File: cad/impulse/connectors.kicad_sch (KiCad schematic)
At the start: 29 parts, among them J1 Screw_Terminal_01x02, J10 Screw_Terminal_01x02, J2 Screw_Terminal_01x02, J3 Conn_01x08, J4 Conn_01x08, J5 Conn_01x08, J6 Screw_Terminal_01x02, J7 GT-USB-7010ASV, J8 Screw_Terminal_01x02, J9 Screw_Terminal_01x02, Q2 Q_NMOS_DGS, Q3 Q_NMOS_DGS, Q4 Q_NMOS_DGS, Q5 Q_NMOS_DGS, U3 USBLC6-2SC6

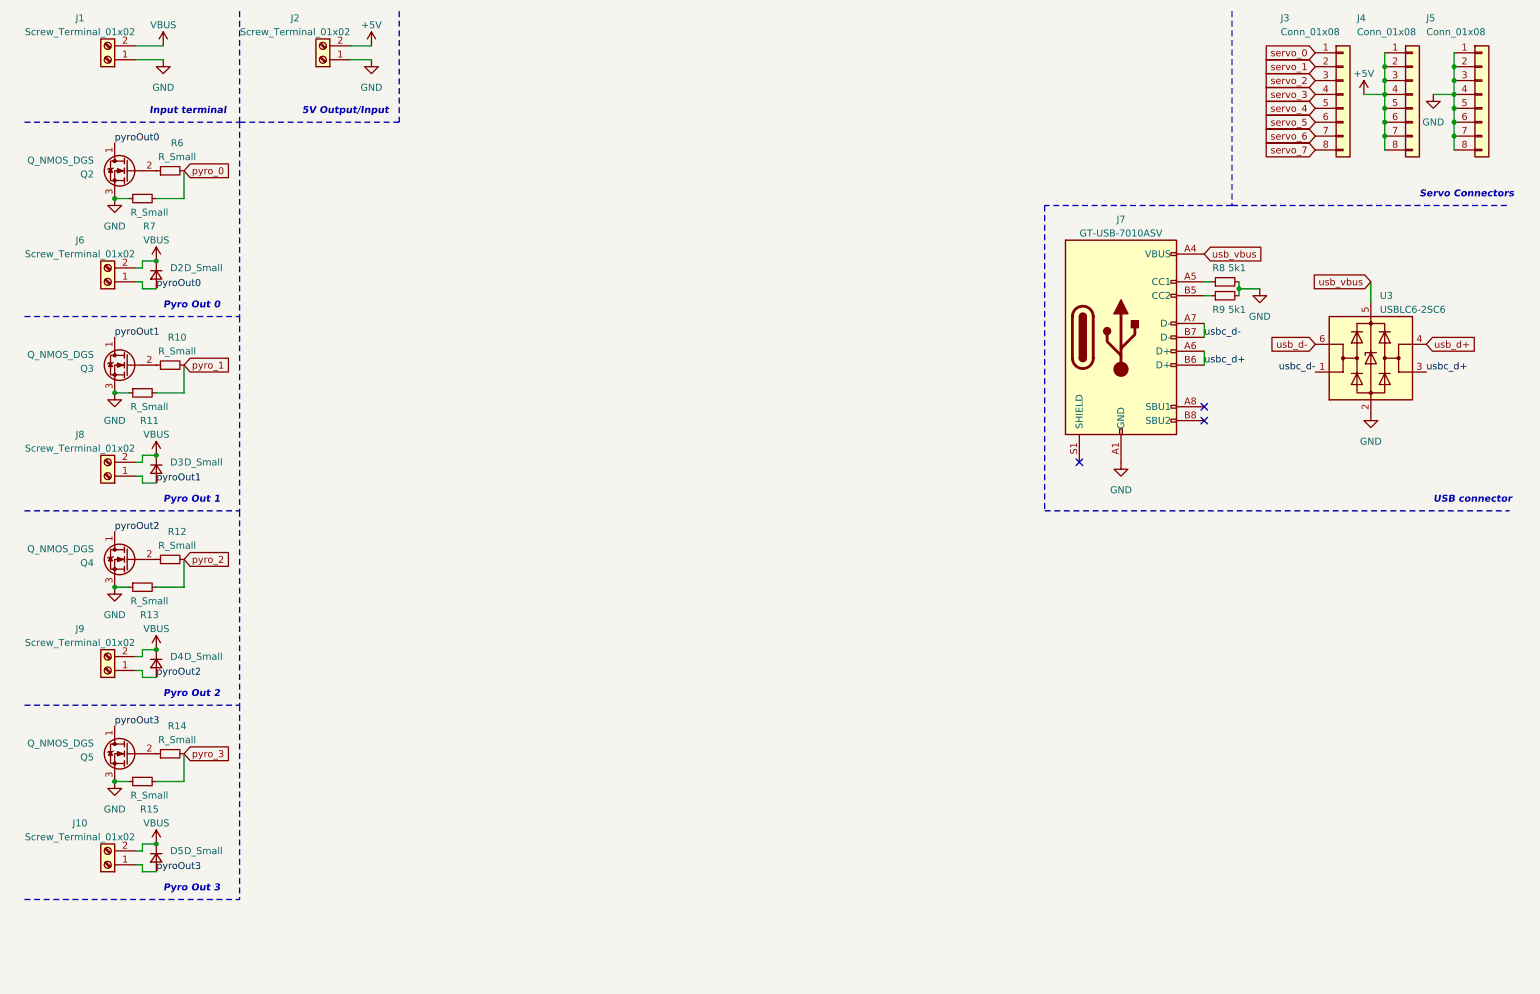
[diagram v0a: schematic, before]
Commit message: Finnished the design.
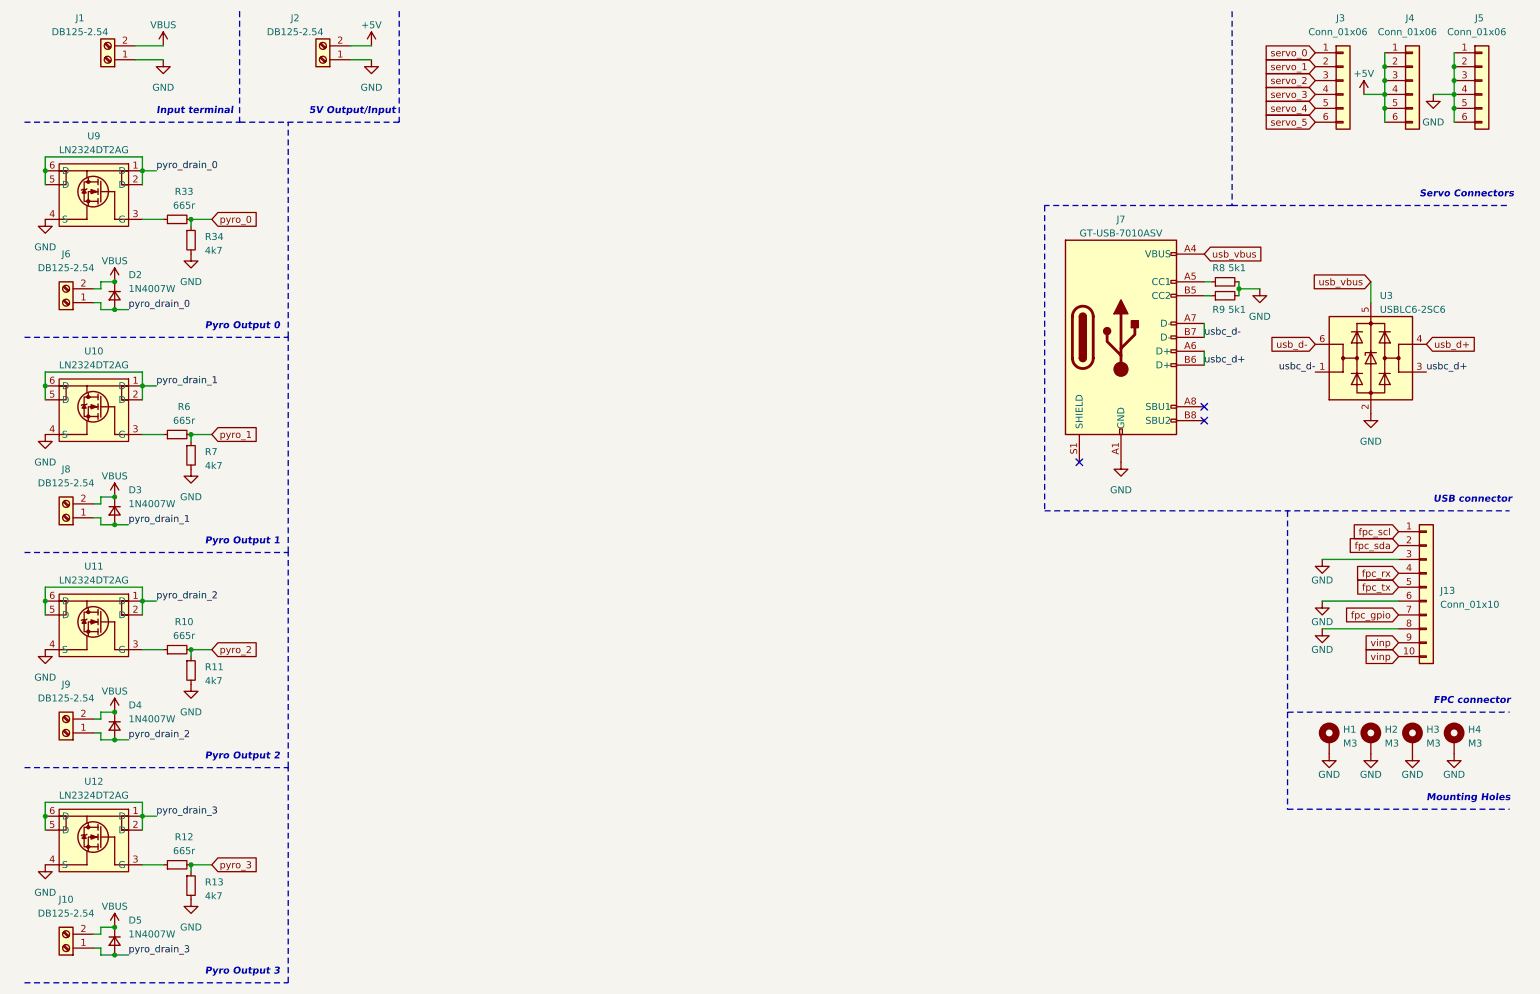
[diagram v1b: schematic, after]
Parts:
- removed J3, J4, J5: Conn_01x08, Connector_RJ:RJ45_Amphenol_54602-x08_Horizontal, symbol Connector_Generic:Conn_01x08
- removed Q2, Q3, Q4, Q5: Q_NMOS_DGS, symbol Device:Q_NMOS_DGS
- removed R14, R15: R_Small, symbol Device:R_Small
- added H1, H2, H3, H4: M3, symbol Mechanical:MountingHole_Pad
- added J13: Conn_01x10, symbol Connector_Generic:Conn_01x10
- added J3, J4, J5: Conn_01x06, symbol Connector_Generic:Conn_01x06
- added R33: 665r, symbol Device:R_Small
- added R34: 4k7, symbol Device:R_Small
- added U10, U11, U12, U9: LN2324DT2AG, symbol impulse:LN2324DT2AG
- D2, D3, D4, D5: value D_Small -> 1N4007W
- J1, J10, J2, J6, J8, J9: value Screw_Terminal_01x02 -> DB125-2.54
- R10, R12, R6: value R_Small -> 665r
- R11, R13, R7: value R_Small -> 4k7
- U3: footprint Package_TO_SOT_SMD:SOT-23-6 -> (none)
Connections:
- net +5V: now also J4.1 (Pin_1), J4.2 (Pin_2), J4.3 (Pin_3), J4.4 (Pin_4), J4.5 (Pin_5), J4.6 (Pin_6)
- net GND: now also R11.2, R13.2, R7.2, H1.1, H2.1, H3.1, H4.1, J13.3 (Pin_3), J13.6 (Pin_6), J13.8 (Pin_8), J5.1 (Pin_1), J5.2 (Pin_2), J5.3 (Pin_3), J5.4 (Pin_4), J5.5 (Pin_5), J5.6 (Pin_6), R34.2, U10.4 (S), U11.4 (S), U12.4 (S), U9.4 (S); no longer R11.1, R13.1, R7.1
- net pyro_0: now also R33.2, R34.1; no longer R6.2, R7.2
- net pyro_1: now also R6.2, R7.1; no longer R10.2, R11.2
- net pyro_2: now also R10.2, R11.1; no longer R12.2, R13.2
- net pyro_3: now also R12.2, R13.1
- net servo_0: now also J3.1 (Pin_1)
- net servo_1: now also J3.2 (Pin_2)
- net servo_2: now also J3.3 (Pin_3)
- net servo_3: now also J3.4 (Pin_4)
- net servo_4: now also J3.5 (Pin_5)
- net servo_5: now also J3.6 (Pin_6)
- net at R12.1: now also U12.3 (G)
- net at R10.1: now also U11.3 (G)
- net at R6.1: now also U10.3 (G)
- net pyroOut0 renamed pyro_drain_0
- net pyro_drain_0: now also U9.1 (D), U9.2 (D), U9.5 (D), U9.6 (D)
- net pyroOut1 renamed pyro_drain_1
- net pyro_drain_1: now also U10.1 (D), U10.2 (D), U10.5 (D), U10.6 (D)
- net pyroOut2 renamed pyro_drain_2
- net pyro_drain_2: now also U11.1 (D), U11.2 (D), U11.5 (D), U11.6 (D)
- net pyroOut3 renamed pyro_drain_3
- net pyro_drain_3: now also U12.1 (D), U12.2 (D), U12.5 (D), U12.6 (D)
- new net: R33.1, U9.3 (G)
- new net fpc_gpio: J13.7 (Pin_7)
- new net fpc_rx: J13.4 (Pin_4)
- new net fpc_scl: J13.1 (Pin_1)
- new net fpc_sda: J13.2 (Pin_2)
- new net fpc_tx: J13.5 (Pin_5)
- new net vinp: J13.10 (Pin_10), J13.9 (Pin_9)
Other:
- note added: "FPC connector"
- note added: "Mounting Holes"
- note added: "Pyro Output 0"
- note added: "Pyro Output 1"
- note added: "Pyro Output 2"
- note added: "Pyro Output 3"
- note removed: "Pyro Out 0"
- note removed: "Pyro Out 1"
- note removed: "Pyro Out 2"
- note removed: "Pyro Out 3"
- company: (none) -> markbel
- title: (none) -> Connectors
- moved on the sheet: D2, J6
